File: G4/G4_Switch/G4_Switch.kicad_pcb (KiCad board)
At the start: 2 copper layers, 70.5 x 91.4 mm, 28 parts, among them J1 Conn_01x09_Socket, J2 Conn_01x09_Socket, J3 DB25_Plug, U1 NUCLEO-G491RE, U2 74HC594, U3 74HC594, U4 ULN2003A, U5 ULN2003A

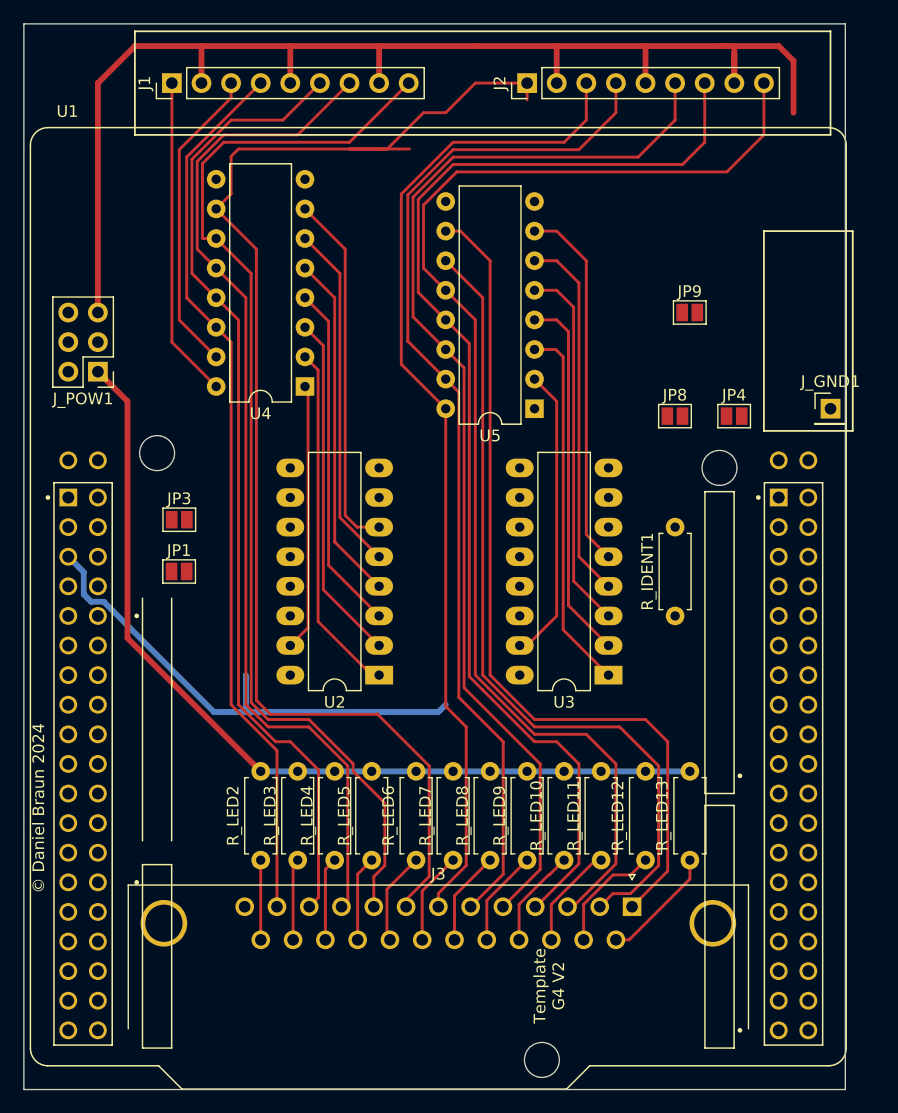
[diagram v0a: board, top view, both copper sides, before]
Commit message: updated G4_Switch
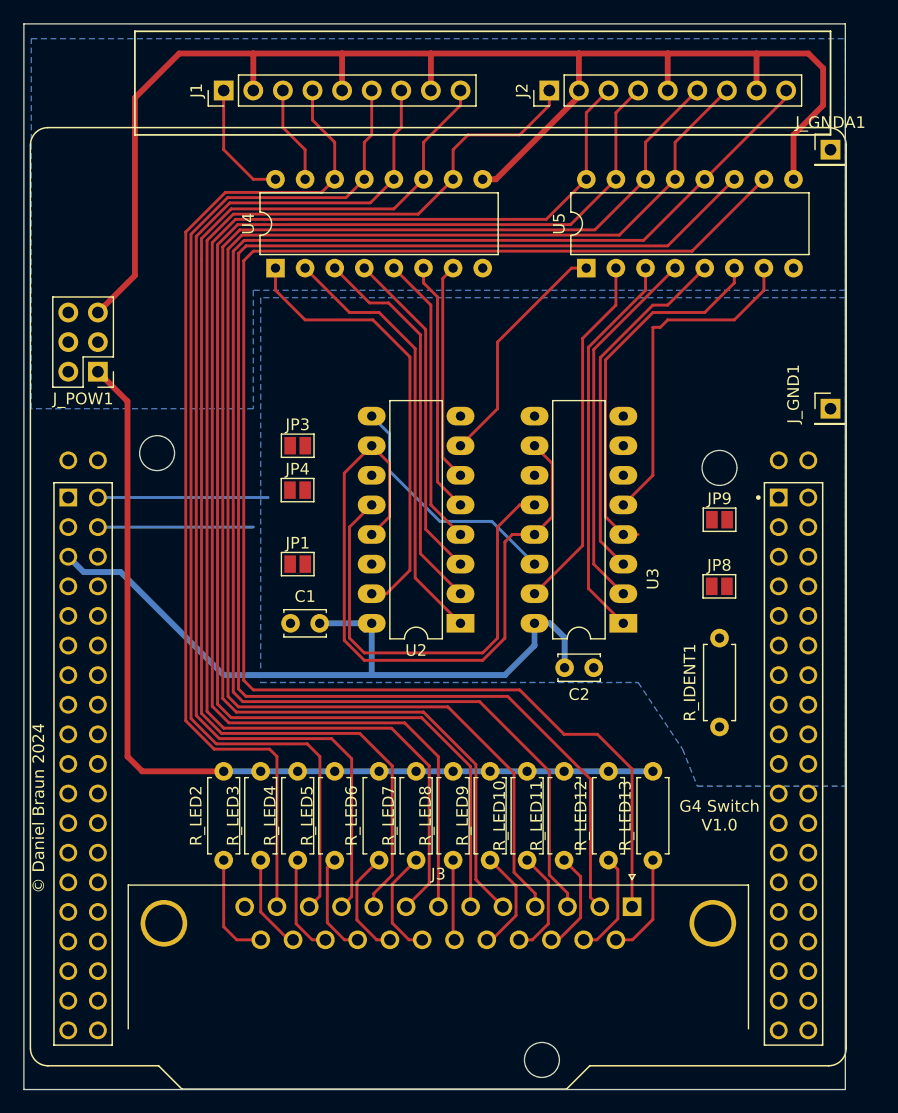
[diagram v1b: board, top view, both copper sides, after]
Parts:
- added C1: C, Capacitor_THT:C_Disc_D3.4mm_W2.1mm_P2.50mm, F.Cu at (115.0, 95.2)
- added C2: C, Capacitor_THT:C_Disc_D3.4mm_W2.1mm_P2.50mm, F.Cu at (141.0, 99.1)
- added J_GNDA1: Conn_01x01_Female, Connector_PinHeader_2.54mm:PinHeader_1x01_P2.54mm_Vertical, F.Cu at (161.3, 54.6)
- U1: footprint G4Lib:MODULE_NUCLEO-G491RE20 -> G4Lib:MODULE_NUCLEO-G491RE20noar
- moved JP4 38.0 mm to (115.6, 83.8)
- moved JP9 18.0 mm to (151.8, 86.4)
- moved JP8 15.1 mm to (151.8, 92.1)
- moved U5 12.9 mm to (140.3, 64.8), turned to 90 degrees
- moved JP3 12.0 mm to (115.6, 80.0)
- moved U4 10.5 mm to (113.7, 64.8), turned to 90 degrees
- moved JP1 10.2 mm to (115.6, 90.2)
- moved U2 8.28 mm to (129.5, 95.2)
- moved U3 4.62 mm to (143.5, 95.2)
- moved J1 4.49 mm to (109.2, 49.5)
- moved R_IDENT1 4.26 mm to (151.8, 96.5), turned to -90 degrees
- moved R_LED10 3.18 mm to (135.3, 115.6)
- moved R_LED4 3.18 mm to (115.6, 115.6)
- moved R_LED8 3.18 mm to (128.9, 115.6)
- moved R_LED2 3.17 mm to (109.2, 115.6)
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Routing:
- net S_CLR: track 0.00 -> 75.1 mm
- net GS13: track 73.5 -> 131.8 mm
- net GS12: track 70.3 -> 127.2 mm
- net S_VALID: track 0.00 -> 54.1 mm
- net GS8: track 88.9 -> 120.3 mm
- net GS7: track 86.1 -> 116.6 mm
- net GS9: track 95.1 -> 124.1 mm
- net GS10: track 100.8 -> 128.2 mm
- net GS11: track 107.8 -> 133.6 mm
- net Net-(U2-QH'): track 0.00 -> 21.1 mm
- net Net-(U2-QH): track 0.00 -> 20.5 mm
- net 3V3: track 42.5 -> 62.7 mm
- net GS1: track 26.6 -> 8.41 mm
- net GS0: track 27.6 -> 9.94 mm
- net Net-(U2-QA): track 23.0 -> 38.2 mm
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- added copper zone on B.Cu, net GND
- added copper zone on B.Cu, net GNDA
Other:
- board text added: "G4 Switch V1.0"
- board text removed: "Template G4 V2"
